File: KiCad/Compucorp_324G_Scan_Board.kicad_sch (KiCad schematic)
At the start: 29 parts, among them J1 Scan Interboard, J2 Power In, J4 From Keyboard, U1 BR 16252, U2 UHP480, U21 TMC1884 (TCL08), U3 UHP480, U4 TMC1869 (TCL02)

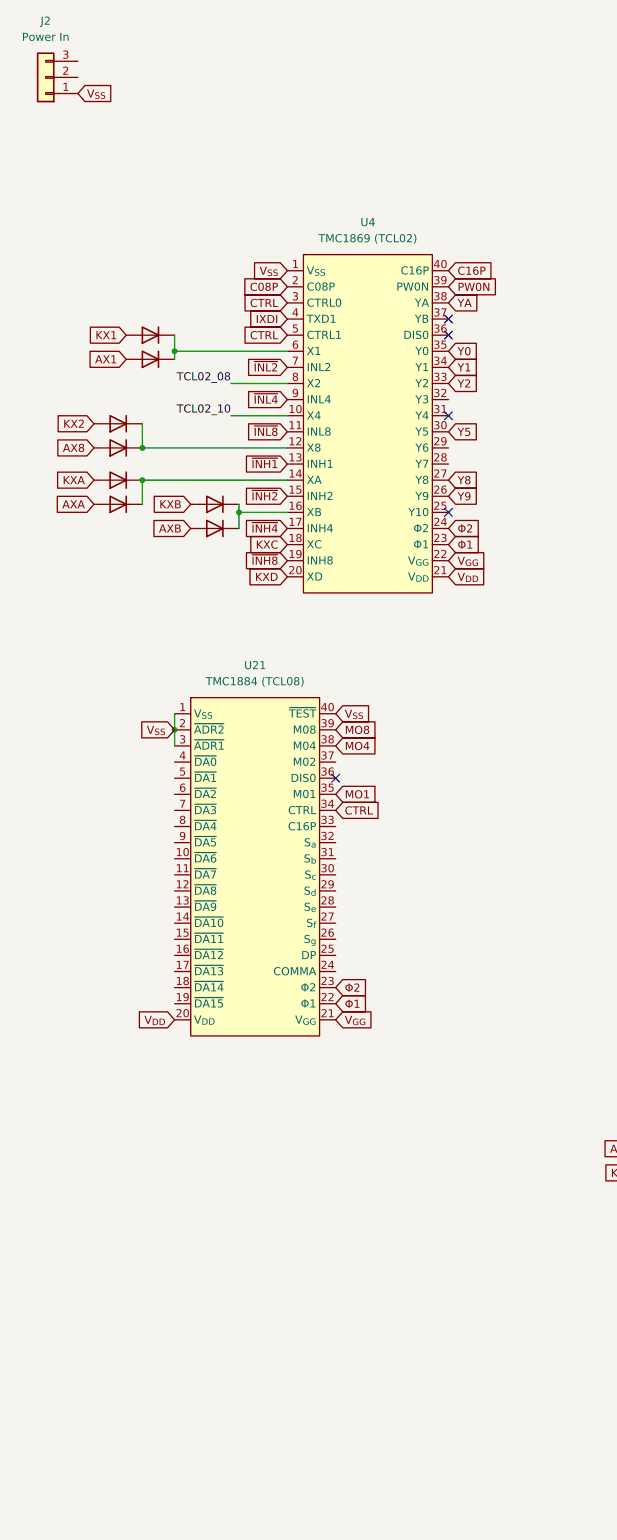
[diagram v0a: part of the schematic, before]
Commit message: Update Compucorp_324G_Scan_Board.kicad_sch
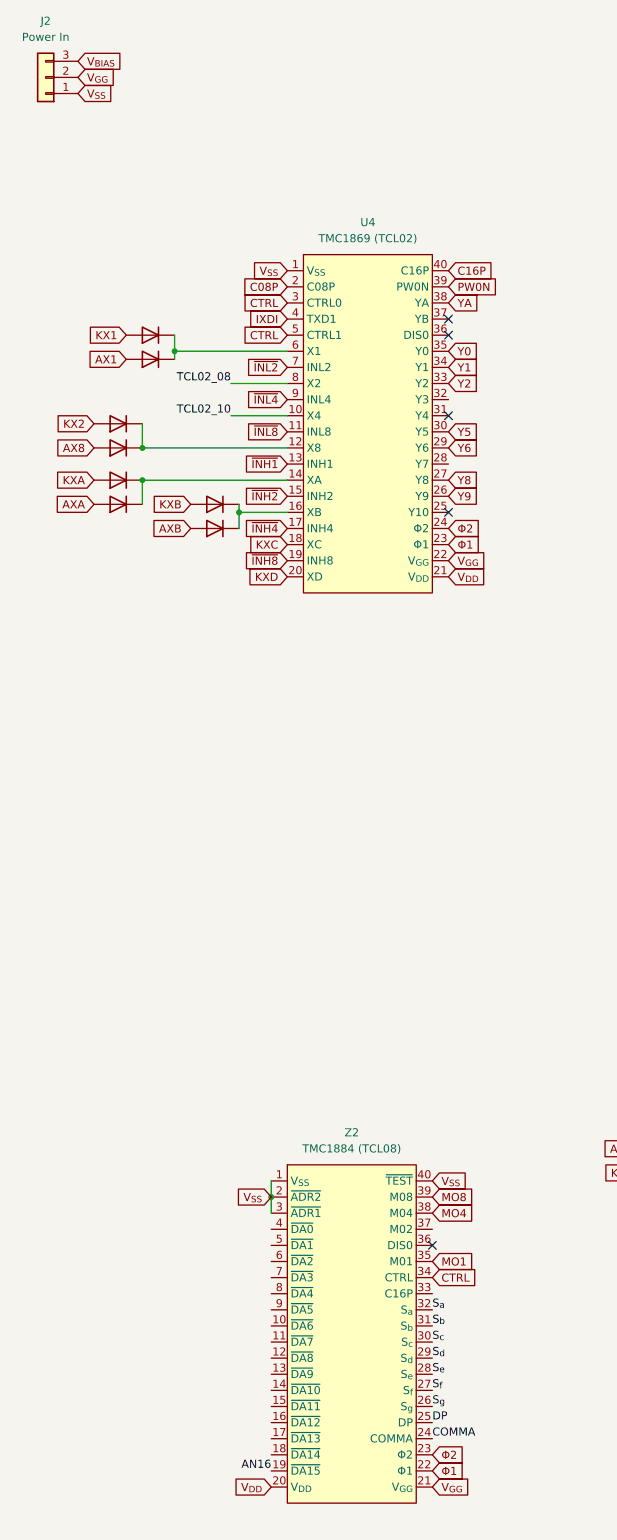
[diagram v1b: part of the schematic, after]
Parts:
- renumbered U21 to Z2
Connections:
- net AN16: now also Z2.19 (~{DA15})
- net COMMA: now also Z2.24 (COMMA)
- net DP: now also Z2.25 (DP)
- net S_{a}: now also Z2.32 (S_{a})
- net S_{b}: now also Z2.31 (S_{b})
- net S_{c}: now also Z2.30 (S_{c})
- net S_{d}: now also Z2.29 (S_{d})
- net S_{e}: now also Z2.28 (S_{e})
- net S_{f}: now also Z2.27 (S_{f})
- net S_{g}: now also Z2.26 (S_{g})
- net V_{GG}: now also J2.2 (Pin_2)
- net Y6: now also U4.29 (Y6)
- net V_{BIAS}: now reaches J2.3 (Pin_3)
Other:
- moved on the sheet: Z2
